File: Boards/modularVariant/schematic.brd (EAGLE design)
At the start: 93 x 70 mm, 93 parts, among them IC1 LM2596S, J1 AVR_SPI_PRG_6NS, Q1 FC-12M, U1 MAGJACK-POE, U2 MAGJACK-POE

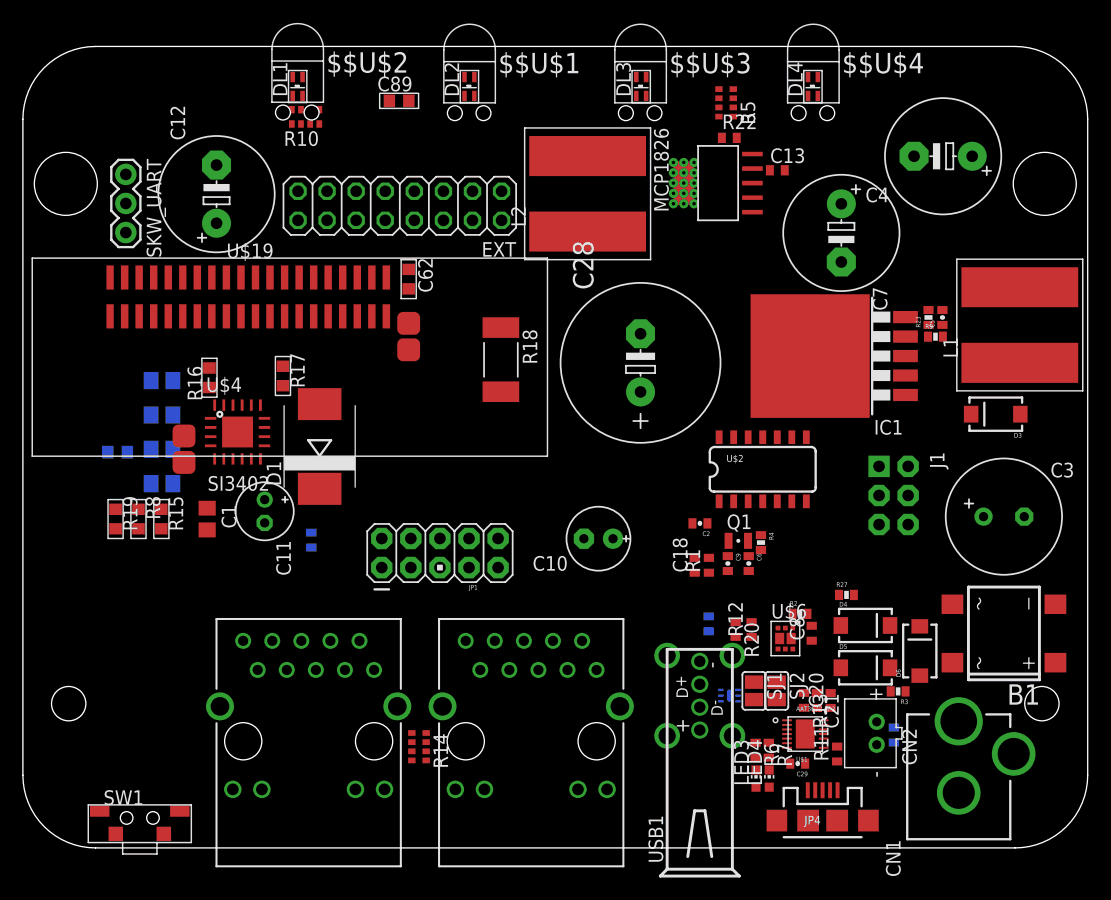
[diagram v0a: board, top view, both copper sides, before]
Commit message: normal Push.
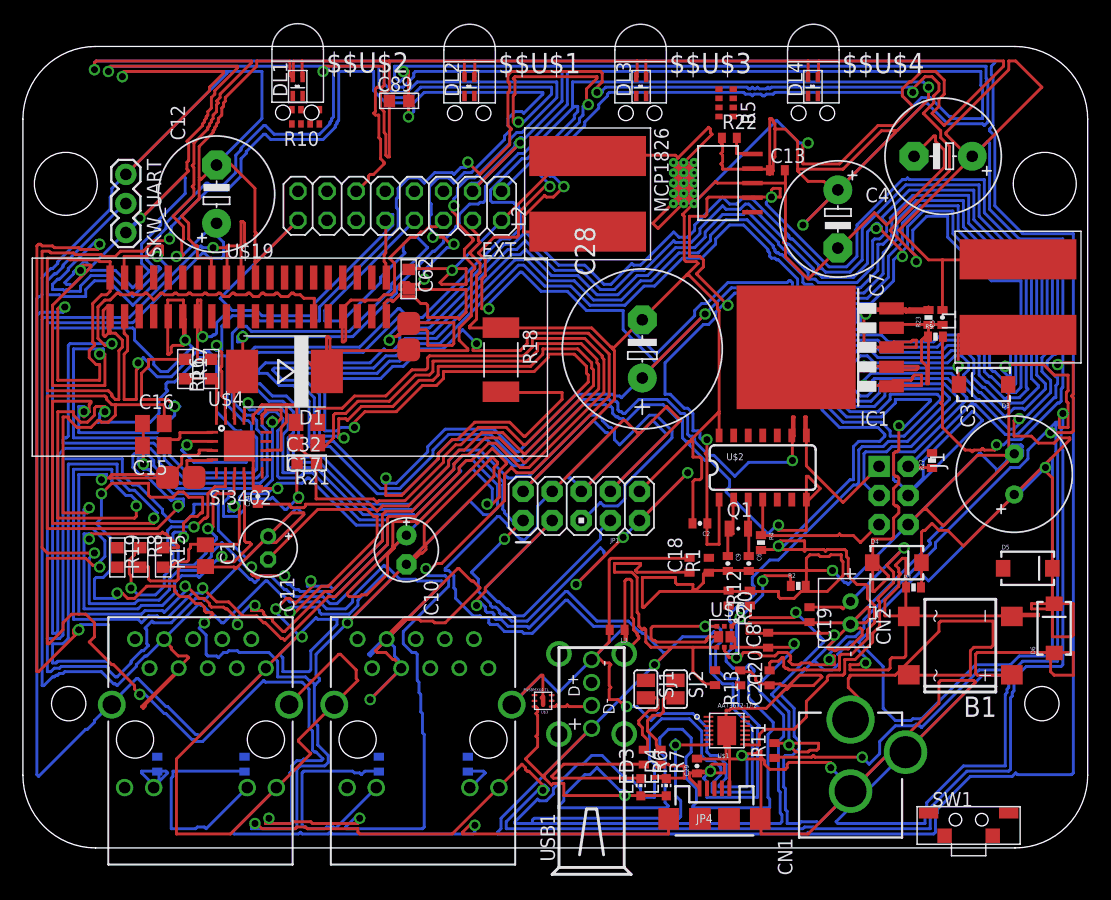
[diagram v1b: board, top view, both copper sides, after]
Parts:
- added R24, R25, R26: 330, SparkFun-Passives:0402-RES
- R14: device SparkFun-Passives:0603-ARV -> SparkFun-Passives:0402-RES
- moved SW1 72.4 mm to (82.6, 1.07)
- moved C10 16.8 mm to (33.5, 26.0), turned to 270 degrees
- moved D5 16.6 mm to (87.8, 24.4)
- moved R21 16.6 mm to (24.8, 33.7), flipped to the top
- moved U$3 16.3 mm to (45.4, 12.8), flipped to the top
- moved R27 13.9 mm to (79.4, 33.8), turned to 90 degrees
- moved C17 13.8 mm to (24.8, 35.4), flipped to the top, turned to 180 degrees
- moved JP1 13.0 mm to (48.8, 29.9)
- moved C19 12.8 mm to (68.7, 20.4), flipped to the top
- moved C32 12.7 mm to (24.8, 37.2), flipped to the top, turned to 180 degrees
- moved D6 11.9 mm to (90.1, 19.2)
- moved CN2 10.8 mm to (72.3, 20.5)
- moved LED3 10.1 mm to (54.0, 5.30)
- moved R6 9.77 mm to (54.2, 7.93)
- moved R7 9.47 mm to (55.7, 7.93)
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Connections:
- net ETH0_GRN+: now also R24.2; no longer R14.4
- net GND: now also R26.1; no longer R14.3
- net N$24: now also R14.1; no longer R14.6
- net N$25: now also R25.2; no longer R14.1
- net N$31: now also R26.2; no longer R14.7
- net N$95: now also R24.1; no longer R14.5
- net VDD: now also R25.1; no longer R14.8
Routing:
- net GND: track 0.00 -> 1490.6 mm, vias 0 -> 18
- net VCC: track 0.00 -> 784.4 mm, vias 0 -> 7
- net VDD: track 0.00 -> 614.0 mm, vias 0 -> 16
- net PD_VDC: track 0.00 -> 536.7 mm, vias 0 -> 15
- net ETH0_GRN-: track 0.00 -> 496.4 mm, vias 0 -> 17
- net +57: track 0.00 -> 370.0 mm, vias 0 -> 4
- net N$6: track 0.00 -> 330.6 mm, vias 0 -> 10
- net VIN: track 0.00 -> 329.4 mm, vias 0 -> 3
- net PA6: track 0.00 -> 250.7 mm, vias 0 -> 1
- net PA4: track 0.00 -> 220.2 mm, vias 0 -> 1
- net VSOURCE: track 0.00 -> 217.5 mm, vias 0 -> 8
- net VLITHIUM: track 0.00 -> 203.3 mm, vias 0 -> 4
- net PD3/TXD: track 0.00 -> 187.7 mm, vias 0 -> 6
- net N$15: track 0.00 -> 175.3 mm, vias 0 -> 4
- net +2V: track 0.00 -> 169.7 mm, vias 0 -> 2
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
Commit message: normal Push.
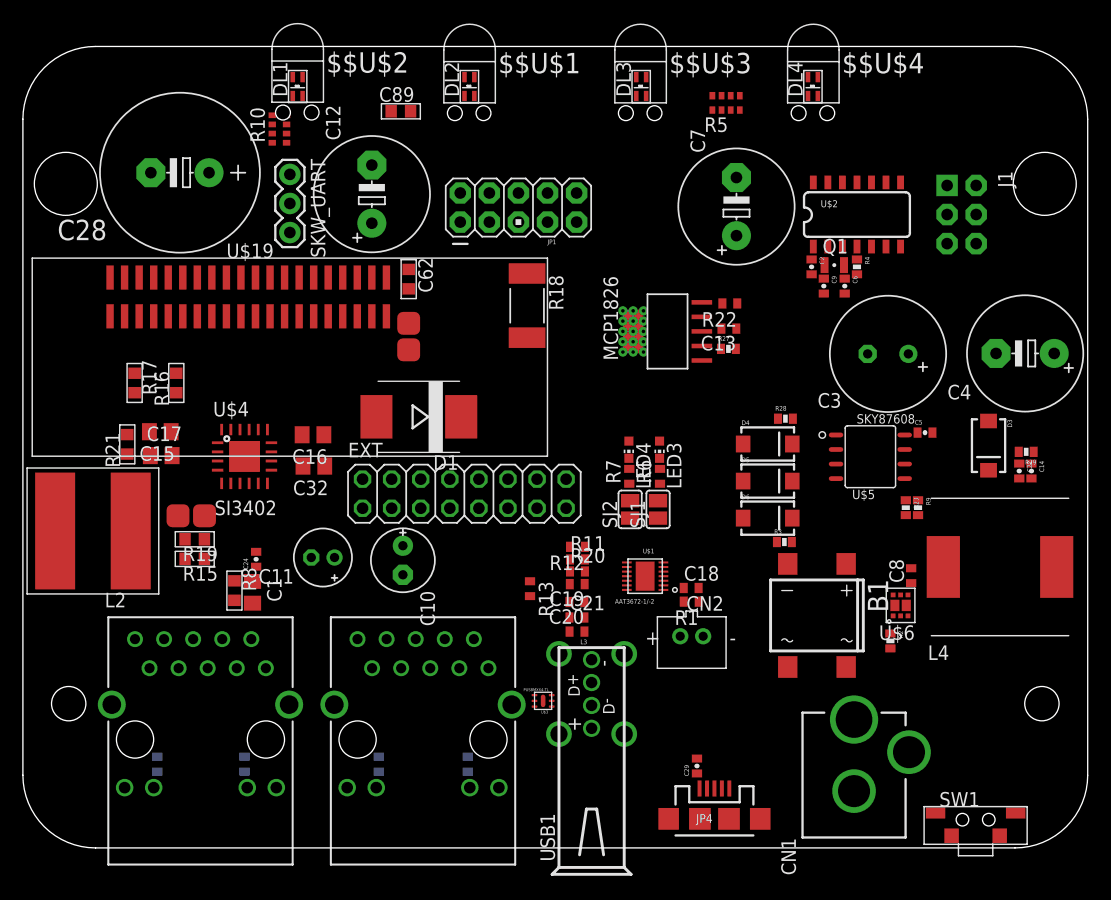
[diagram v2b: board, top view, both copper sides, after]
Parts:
- removed IC1: LM2596S, national-semiconductor:TO263-5
- removed L1: 33uH 3A, schematic:INDUCTOR-10X9.8X6
- added C14: 56pF, SparkFun-Capacitors:0402-CAP
- added C22: 10nF, SparkFun-Capacitors:0402-CAP
- added L4: 6.8uH, WE-PD:WE-PD_1260/1245/1280/1210
- added R28: 100k, SparkFun-Passives:0402-RES
- added R29: 3k, SparkFun-Passives:0402-RES
- added U$5: SKY87608, schematic:8PIN-SOP-8L-EP
- C5: value (none) -> 0.1uF
- R23: value 3.2k -> 20k
- R9: value 1k -> 91k
- moved L2 52.3 mm to (6.12, 27.7), turned to 180 degrees
- moved C28 43.2 mm to (13.7, 59.0), turned to 180 degrees
- moved LED4 29.7 mm to (52.9, 34.8), turned to 180 degrees
- moved LED3 29.5 mm to (55.6, 34.8), turned to 180 degrees
- moved D6 26.8 mm to (65.1, 28.8), turned to 0 degrees
- moved JP1 26.6 mm to (43.3, 55.9)
- moved EXT 25.8 mm to (38.6, 30.9), turned to 0 degrees
- moved C6 25.6 mm to (71.8, 49.1)
- moved C9 25.6 mm to (70.0, 49.1)
- moved R4 25.5 mm to (72.8, 50.7)
- moved J1 25.2 mm to (82.0, 55.3)
- moved R7 24.7 mm to (53.0, 32.5), turned to 90 degrees
- moved R6 24.6 mm to (55.6, 32.5), turned to 90 degrees
- moved Q1 24.5 mm to (70.9, 50.9)
- moved C2 24.4 mm to (68.9, 50.7), turned to 270 degrees
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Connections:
- new net CMP: C14.2, C22.2, U$5.P$6
- new net N$22: R28.1, U$5.P$7
- new net N$27: R23.1, R9.1, U$5.P$5
- new net N$37: C22.1, R29.2
- net GND: now also C14.1, R29.1, U$5.P$4; no longer EXT.10, EXT.16, IC1.3, IC1.5
- net GPIO_23: now also EXT.11; no longer EXT.15
- net N$2: now also C5.2, L4.1, U$5.P$2; no longer IC1.2, L1.P$1
- net N$26: now also U$5.P$8; no longer IC1.4, R23.1, R9.1
- net PA0: now also SJ2.1; no longer R5.3
- net PA1: now also SJ1.1; no longer R5.4
- net PA4: no longer SJ1.1
- net PA5: now also R5.3
- net PA6: now also R5.4; no longer SJ2.1
- net PD3/TXD: now also EXT.10; no longer EXT.11
- net USB_D_N: now also EXT.16
- net USB_D_P: now also EXT.15
- net VIN: now also R28.2, U$5.P$1; no longer IC1.1
- net VSOURCE: now also L4.2; no longer C5.2, L1.P$2
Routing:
- net GND: track 1490.6 -> 0.00 mm, vias 18 -> 0
- net VCC: track 784.4 -> 0.00 mm, vias 7 -> 0
- net VDD: track 614.0 -> 0.00 mm, vias 16 -> 0
- net PD_VDC: track 536.7 -> 0.00 mm, vias 15 -> 0
- net ETH0_GRN-: track 496.4 -> 0.00 mm, vias 17 -> 0
- net +57: track 370.0 -> 0.00 mm, vias 4 -> 0
- net N$6: track 330.6 -> 0.00 mm, vias 10 -> 0
- net VIN: track 329.4 -> 0.00 mm, vias 3 -> 0
- net PA6: track 250.7 -> 0.00 mm, vias 1 -> 0
- net PA4: track 220.2 -> 0.00 mm, vias 1 -> 0
- net VSOURCE: track 217.5 -> 0.00 mm, vias 8 -> 0
- net VLITHIUM: track 203.3 -> 0.00 mm, vias 4 -> 0
- net PD3/TXD: track 187.7 -> 0.00 mm, vias 6 -> 0
- net N$15: track 175.3 -> 0.00 mm, vias 4 -> 0
- net +2V: track 169.7 -> 0.00 mm, vias 2 -> 0
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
